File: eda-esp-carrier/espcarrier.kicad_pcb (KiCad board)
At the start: 2 copper layers, 38.5 x 38.5 mm, 22 parts, among them J1 BATT, J3 DEBUG, Q1 PMF170XP, Q2 DMN2310U, SW1 PWR, SW2 RST, SW3 PRGM, U1 TP4056_board, U2 ESP-12E, U3 TLV75533PDBV

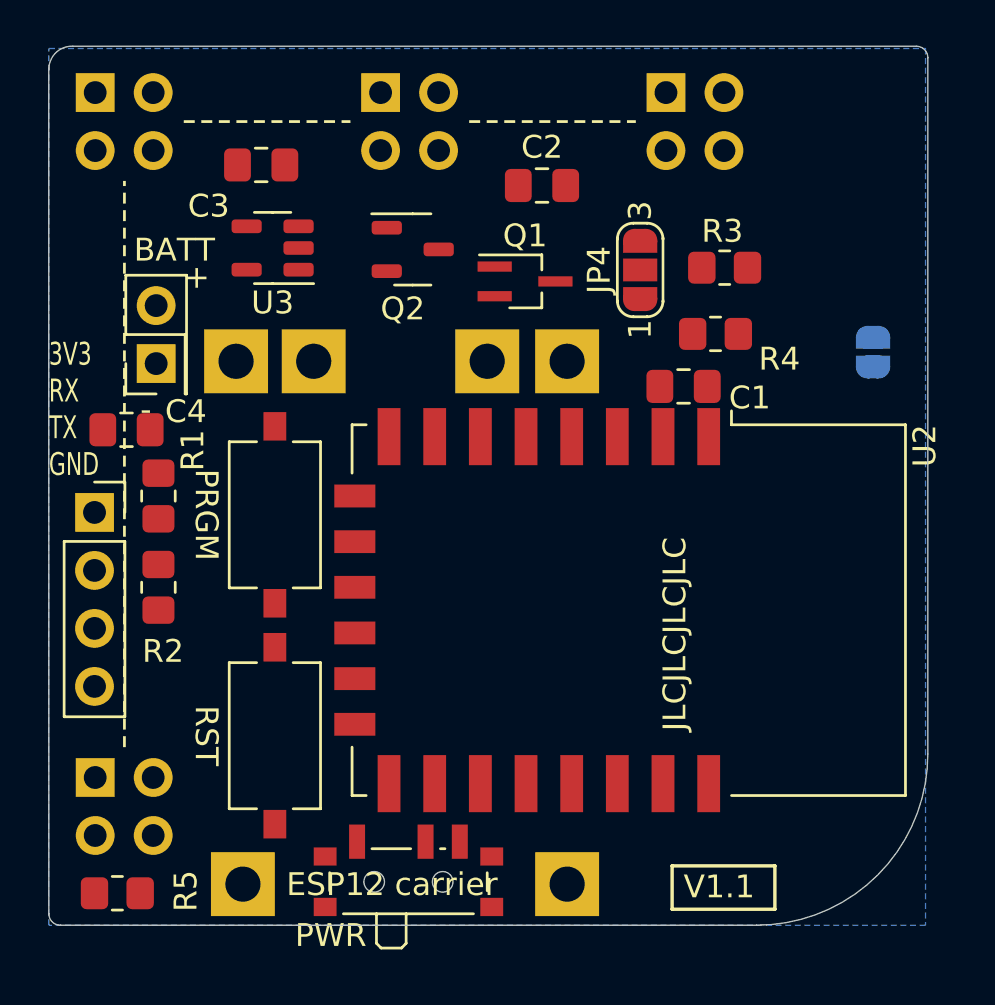
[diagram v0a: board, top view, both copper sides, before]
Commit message: finish rf friendlier desgin
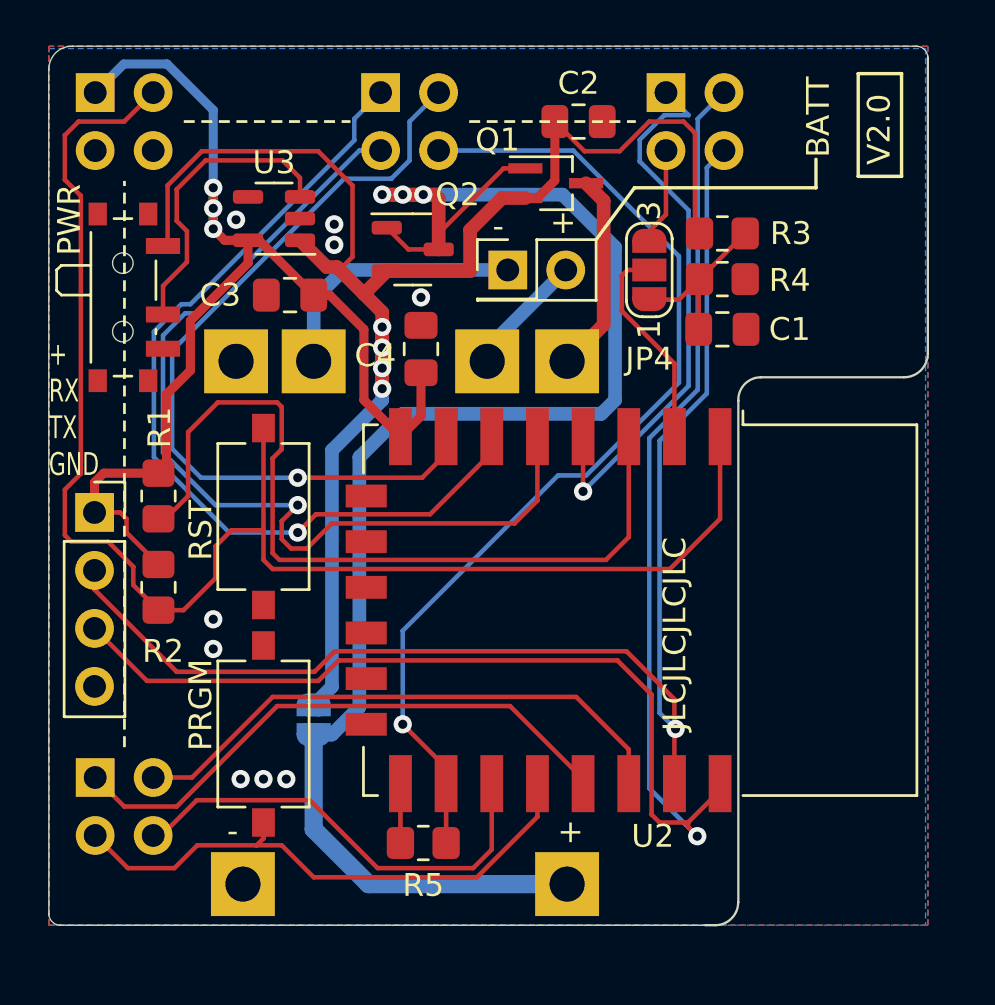
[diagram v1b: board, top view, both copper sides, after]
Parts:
- moved JP3 29.3 mm to (67.1, 132.2), turned to 90 degrees
- moved SW1 28.1 mm to (59.1, 113.7), turned to -90 degrees
- moved J1 15.9 mm to (75.6, 112.5), turned to 0 degrees
- moved R5 13.6 mm to (71.9, 137.6), turned to 180 degrees
- moved C4 13.4 mm to (71.8, 116.0), turned to -90 degrees
- moved SW2 9.61 mm to (64.9, 123.3), turned to 90 degrees
- moved SW3 9.61 mm to (64.9, 132.8), turned to 90 degrees
- moved C3 5.84 mm to (66.1, 113.6), turned to 180 degrees
- moved Q1 4.50 mm to (77.7, 108.7)
- moved C2 3.22 mm to (78.7, 106.0)
- moved C1 3.02 mm to (85.0, 115.1)
- moved R4 2.42 mm to (85.0, 112.9)
- moved R3 1.50 mm to (85.0, 110.9)
- moved U3 1.29 mm to (65.4, 110.2)
- moved U2 0.50 mm to (81.4, 127.4)
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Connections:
- net /VIN renamed VIN
- net Net-(J1-Pin_1) renamed /B-
- net Net-(J1-Pin_2) renamed /B+
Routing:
- net Net-(JP3-A): track 0.00 -> 73.0 mm, vias 0 -> 3
- net TXD: track 0.00 -> 71.2 mm, vias 0 -> 1
- net VIN: track 0.00 -> 68.5 mm, vias 0 -> 4
- net ~{RST}: track 0.00 -> 66.0 mm
- net RXD: track 0.00 -> 59.5 mm, vias 0 -> 1
- net +3V3: track 0.00 -> 50.9 mm, vias 0 -> 3
- net GPIO15: track 0.00 -> 44.7 mm, vias 0 -> 1
- net GPIO14: track 0.00 -> 41.9 mm, vias 0 -> 1
- net GPIO12: track 0.00 -> 38.6 mm, vias 0 -> 1
- net Net-(U2-EN): track 0.00 -> 36.3 mm
- net GPIO13: track 0.00 -> 35.4 mm, vias 0 -> 1
- net GPIO4: track 0.00 -> 25.2 mm
- net GPIO5: track 0.00 -> 24.7 mm
- net GPIO0: track 0.00 -> 24.6 mm
- net GPIO16: track 0.00 -> 24.6 mm, vias 0 -> 1
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- added copper zone on F.Cu, net GND
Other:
- outline, holes or cut-outs redrawn
- board text added: "+ RX TX GND"
- board text added: "ESP12-carrier (c) 2024 Andreas Philipp"
- board text added: "V${REVISION}"
- board text added: "https://gitlab.com/ anphi/esp12-battery -breakout"
- board text removed: "3V3 RX TX GND"
- board text removed: "ESP12 carrier"
- board text removed: "ESP12 carrier board https://gitlab.com/anphi/ esp12-battery-breakout (c) 2024 - Andreas Philipp"
- board text removed: "V1.1"
